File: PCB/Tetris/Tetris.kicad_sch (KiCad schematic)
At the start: 49 parts, among them J1 Power, J2 PWM, J3 Analog, J4 PWM, J5 Analog, J6 Communication, J7 Digital, M1 RGBMatrix, M2 RGBMatrix, SW1 SW_Push, SW2 SW_Push, SW3 SW_Push, SW4 SW_Push, SW5 SW_Push, SW6 SW_Push, SW7 SW_Push, U1 74HC595, U2 74HC595

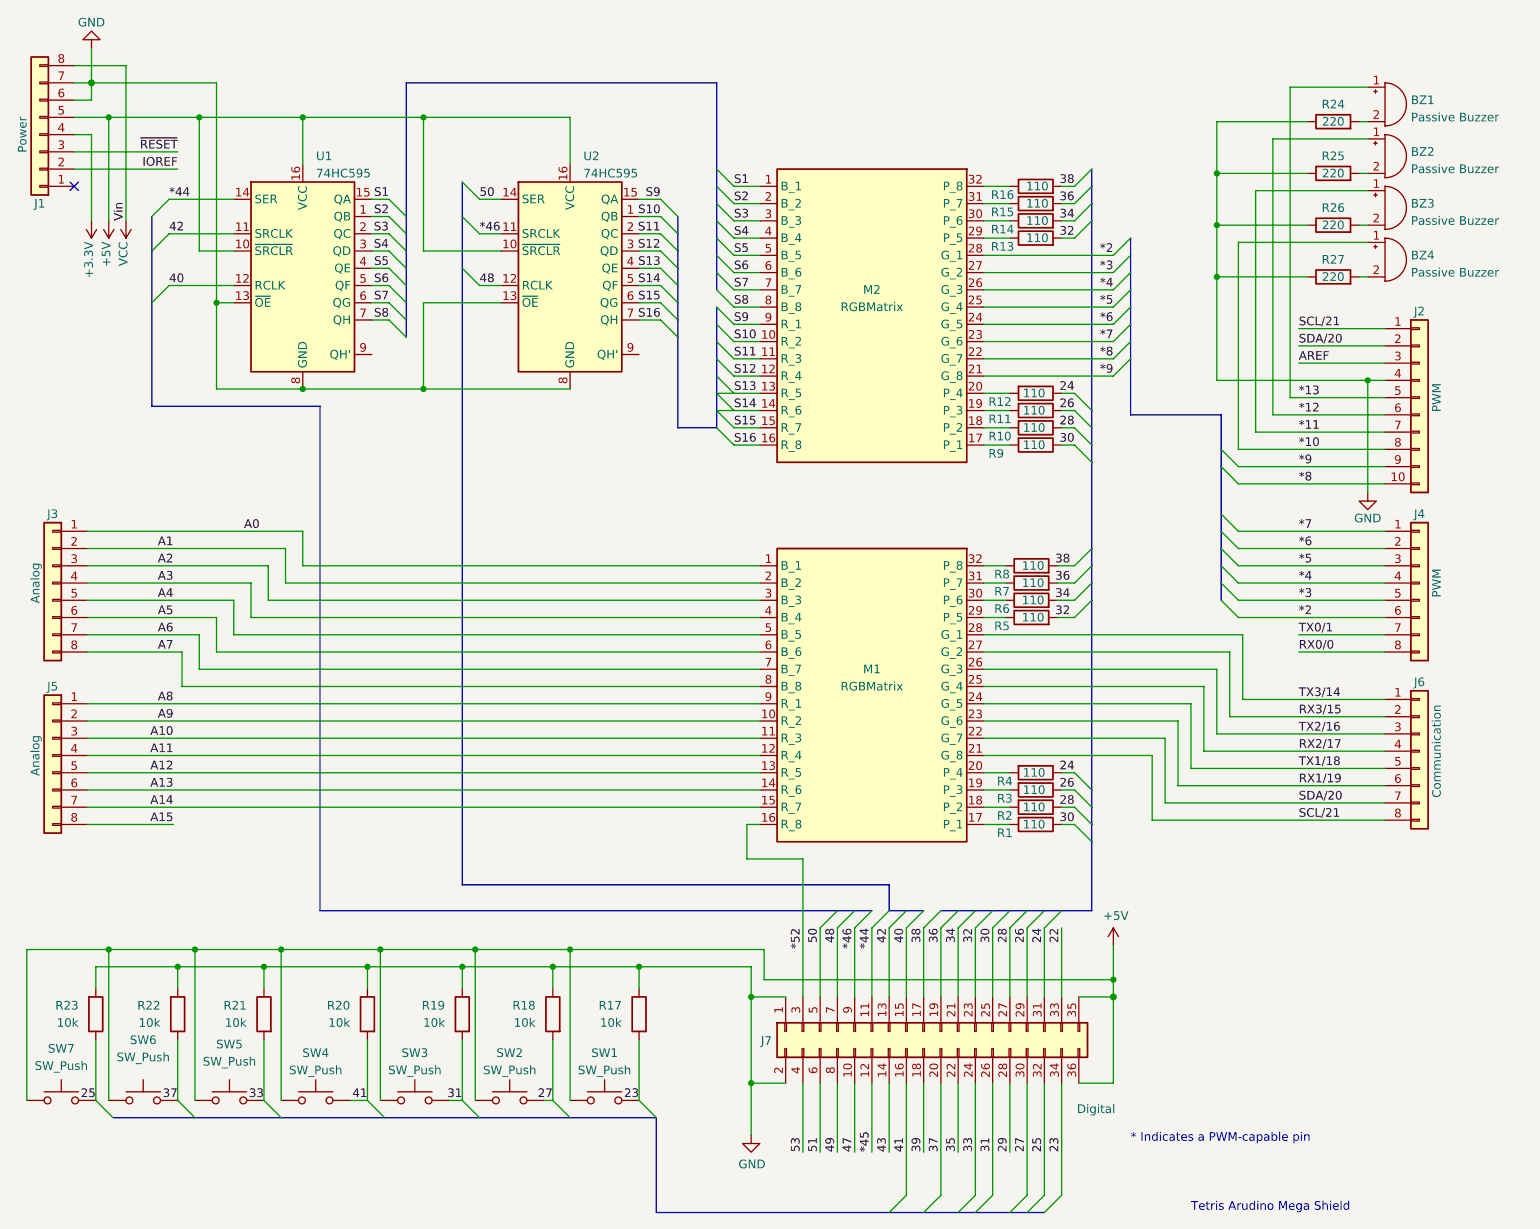
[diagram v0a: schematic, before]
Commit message: sync hcnages
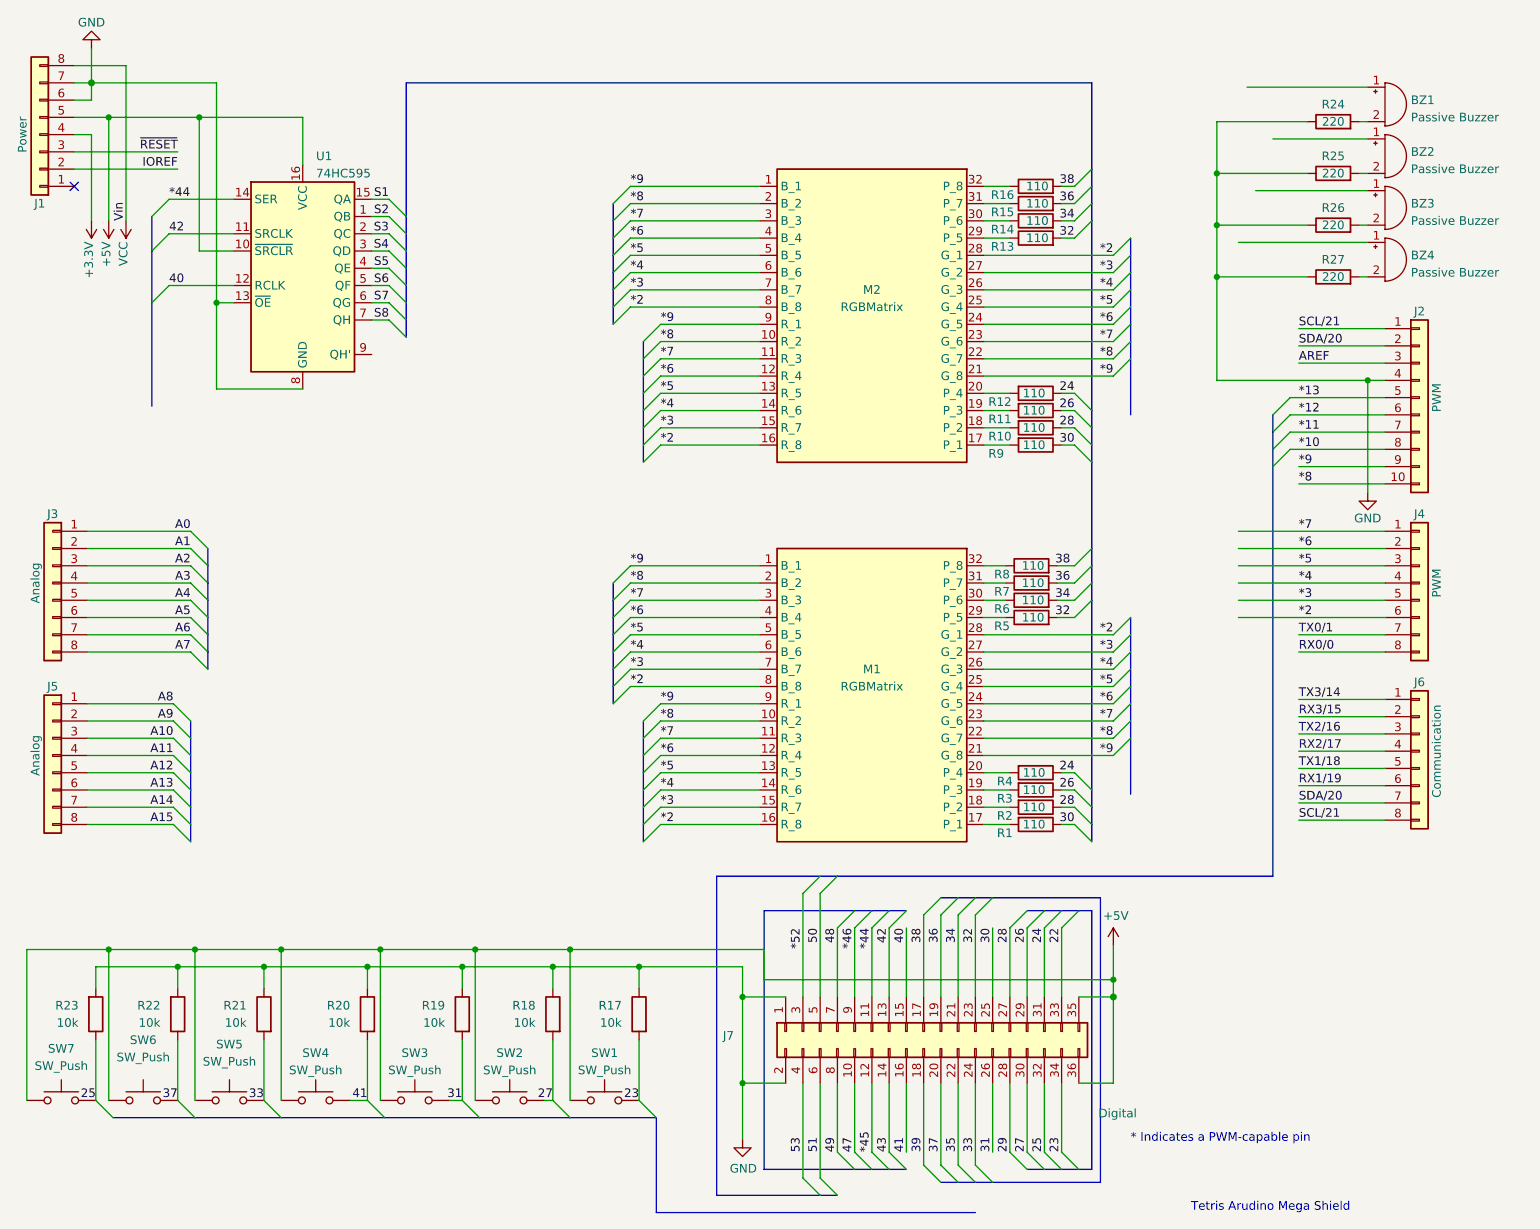
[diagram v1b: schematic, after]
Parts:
- removed U2: 74HC595, Package_DIP:DIP-16_W7.62mm_Socket_LongPads, symbol 74xx:74HC595
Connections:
- net S10 is gone; now on net *8: M2.10 (R_2)
- net S11 is gone; now on net *7: M2.11 (R_3)
- net S12 is gone; now on net *6: M2.12 (R_4)
- net S13 is gone; now on net *5: M2.13 (R_5)
- net S14 is gone; now on net *4: M2.14 (R_6)
- net S15 is gone; now on net *3: M2.15 (R_7)
- net S16 is gone; now on net *2: M2.16 (R_8)
- net S9 is gone; now on net *9: M2.9 (R_1)
- net *10: no longer BZ4.1 (-)
- net *11: no longer BZ3.1 (-)
- net *12: no longer BZ2.1 (-)
- net *13: no longer BZ1.1 (-)
- net *2: now also M1.16 (R_8), M1.28 (G_1), M1.8 (B_8), M2.8 (B_8)
- net *3: now also M1.15 (R_7), M1.27 (G_2), M1.7 (B_7), M2.7 (B_7)
- net *4: now also M1.14 (R_6), M1.26 (G_3), M1.6 (B_6), M2.6 (B_6)
- net *5: now also M1.13 (R_5), M1.25 (G_4), M1.5 (B_5), M2.5 (B_5)
- net *52: no longer M1.16 (R_8)
- net *6: now also M1.12 (R_4), M1.24 (G_5), M1.4 (B_4), M2.4 (B_4)
- net *7: now also M1.11 (R_3), M1.23 (G_6), M1.3 (B_3), M2.3 (B_3)
- net *8: now also M1.10 (R_2), M1.2 (B_2), M1.22 (G_7), M2.2 (B_2)
- net *9: now also M1.1 (B_1), M1.21 (G_8), M1.9 (R_1), M2.1 (B_1)
- net A0: no longer M1.1 (B_1)
- net A1: no longer M1.2 (B_2)
- net A10: no longer M1.11 (R_3)
- net A11: no longer M1.12 (R_4)
- net A12: no longer M1.13 (R_5)
- net A13: no longer M1.14 (R_6)
- net A14: no longer M1.15 (R_7)
- net A2: no longer M1.3 (B_3)
- net A3: no longer M1.4 (B_4)
- net A4: no longer M1.5 (B_5)
- net A5: no longer M1.6 (B_6)
- net A6: no longer M1.7 (B_7)
- net A7: no longer M1.8 (B_8)
- net A8: no longer M1.9 (R_1)
- net A9: no longer M1.10 (R_2)
- net RX1/19: no longer M1.23 (G_6)
- net RX2/17: no longer M1.25 (G_4)
- net RX3/15: no longer M1.27 (G_2)
- net S1: no longer M2.1 (B_1)
- net S2: no longer M2.2 (B_2)
- net S3: no longer M2.3 (B_3)
- net S4: no longer M2.4 (B_4)
- net S5: no longer M2.5 (B_5)
- net S6: no longer M2.6 (B_6)
- net S7: no longer M2.7 (B_7)
- net S8: no longer M2.8 (B_8)
- net SCL/21: no longer M1.21 (G_8)
- net SDA/20: no longer M1.22 (G_7)
- net TX1/18: no longer M1.24 (G_5)
- net TX2/16: no longer M1.26 (G_3)
- net TX3/14: no longer M1.28 (G_1)

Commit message: MASSIVE PROGRESS
Redesign PCB to use ports
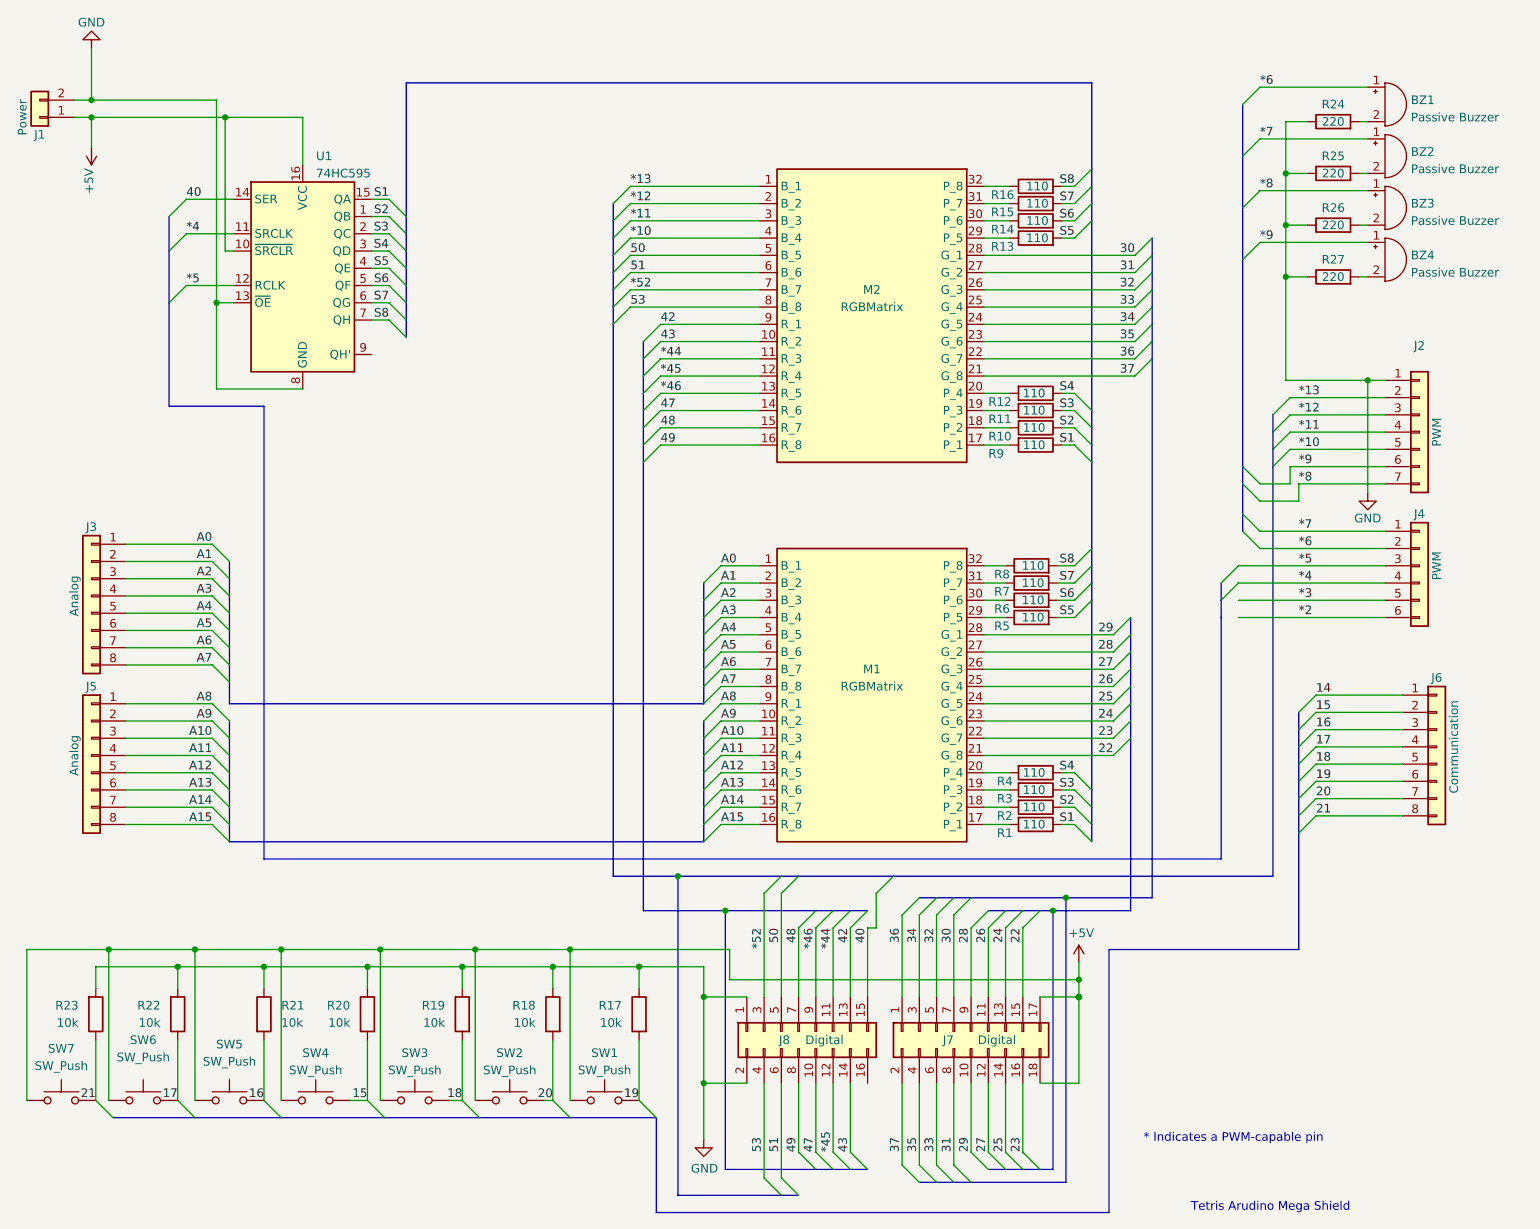
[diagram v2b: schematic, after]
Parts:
- added J8: Digital, Connector_PinHeader_2.54mm:PinHeader_2x08_P2.54mm_Vertical, symbol Connector_Generic:Conn_02x08_Odd_Even
- J1: footprint Connector_PinHeader_2.54mm:PinHeader_1x08_P2.54mm_Vertical -> Connector_PinHeader_2.54mm:PinHeader_1x02_P2.54mm_Vertical; symbol Connector_Generic:Conn_01x08 -> Connector_Generic:Conn_01x02
- J2: footprint Connector_PinHeader_2.54mm:PinHeader_1x10_P2.54mm_Vertical -> Connector_PinHeader_2.54mm:PinHeader_1x07_P2.54mm_Vertical; symbol Connector_Generic:Conn_01x10 -> Connector_Generic:Conn_01x07
- J4: footprint Connector_PinHeader_2.54mm:PinHeader_1x08_P2.54mm_Vertical -> Connector_PinHeader_2.54mm:PinHeader_1x06_P2.54mm_Vertical; symbol Connector_Generic:Conn_01x08 -> Connector_Generic:Conn_01x06
- J7: footprint Connector_PinHeader_2.54mm:PinHeader_2x18_P2.54mm_Vertical -> Connector_PinHeader_2.54mm:PinHeader_2x09_P2.54mm_Vertical; symbol Connector_Generic:Conn_02x18_Odd_Even -> Connector_Generic:Conn_02x09_Odd_Even
- R1, R10, R11, R12, R2, R24, R25, R26, R27, R3, R4, R5, R6, R7, R8, R9: footprint Resistor_THT:R_Axial_DIN0207_L6.3mm_D2.5mm_P10.16mm_Horizontal -> RGBMatrix:R_Axial_DIN0207_L6.3mm_D2.5mm_P12.40mm_Horizontal
- R17, R18: footprint Resistor_THT:R_Axial_DIN0207_L6.3mm_D2.5mm_P10.16mm_Horizontal -> Resistor_THT:R_Axial_DIN0207_L6.3mm_D2.5mm_P7.62mm_Horizontal
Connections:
- net 39 is gone; now on net +5V: J7.18 (Pin_18)
- net AREF is gone; now on net *12: J2.3 (Pin_3)
- net IOREF is gone; now on net GND: J1.2 (Pin_2)
- net RX3/15 is gone; now on net 15: J6.2 (Pin_2)
- net *10: now also J2.5 (Pin_5), M2.4 (B_4); no longer J2.8 (Pin_8)
- net *11: now also J2.4 (Pin_4), M2.3 (B_3); no longer J2.7 (Pin_7)
- net *12: now also M2.2 (B_2); no longer J2.6 (Pin_6)
- net *13: now also J2.2 (Pin_2), M2.1 (B_1); no longer J2.5 (Pin_5)
- net *2: no longer M1.16 (R_8), M1.28 (G_1), M1.8 (B_8), M2.16 (R_8), M2.28 (G_1), M2.8 (B_8)
- net *3: no longer M1.15 (R_7), M1.27 (G_2), M1.7 (B_7), M2.15 (R_7), M2.27 (G_2), M2.7 (B_7)
- net *4: now also U1.11 (SRCLK); no longer M1.14 (R_6), M1.26 (G_3), M1.6 (B_6), M2.14 (R_6), M2.26 (G_3), M2.6 (B_6)
- net *44: now also M2.11 (R_3), J8.11 (Pin_11); no longer J7.11 (Pin_11), U1.14 (SER)
- net *45: now also M2.12 (R_4), J8.12 (Pin_12); no longer J7.12 (Pin_12)
- net *46: now also M2.13 (R_5), J8.9 (Pin_9); no longer J7.9 (Pin_9)
- net *5: now also U1.12 (RCLK); no longer M1.13 (R_5), M1.25 (G_4), M1.5 (B_5), M2.13 (R_5), M2.25 (G_4), M2.5 (B_5)
- net *52: now also M2.7 (B_7), J8.3 (Pin_3); no longer J7.3 (Pin_3)
- net *6: now also BZ1.1 (-); no longer M1.12 (R_4), M1.24 (G_5), M1.4 (B_4), M2.12 (R_4), M2.24 (G_5), M2.4 (B_4)
- net *7: now also BZ2.1 (-); no longer M1.11 (R_3), M1.23 (G_6), M1.3 (B_3), M2.11 (R_3), M2.23 (G_6), M2.3 (B_3)
- net *8: now also BZ3.1 (-), J2.7 (Pin_7); no longer J2.10 (Pin_10), M1.10 (R_2), M1.2 (B_2), M1.22 (G_7), M2.10 (R_2), M2.2 (B_2), M2.22 (G_7)
- net *9: now also BZ4.1 (-), J2.6 (Pin_6); no longer J2.9 (Pin_9), M1.1 (B_1), M1.21 (G_8), M1.9 (R_1), M2.1 (B_1), M2.21 (G_8), M2.9 (R_1)
- net +5V: now also J1.1 (Pin_1), J7.17 (Pin_17); no longer J1.5 (Pin_5), J7.35 (Pin_35), J7.36 (Pin_36)
- net 22: now also J7.15 (Pin_15), M1.21 (G_8); no longer J7.33 (Pin_33)
- net 23: now also J7.16 (Pin_16), M1.22 (G_7); no longer J7.34 (Pin_34), R17.2, SW1.1
- net 24: now also J7.13 (Pin_13), M1.23 (G_6); no longer J7.31 (Pin_31), R12.1, R4.1
- net 25: now also J7.14 (Pin_14), M1.24 (G_5); no longer J7.32 (Pin_32), R23.1, SW7.1
- net 26: now also J7.11 (Pin_11), M1.25 (G_4); no longer J7.29 (Pin_29), R11.1, R3.1
- net 27: now also J7.12 (Pin_12), M1.26 (G_3); no longer J7.30 (Pin_30), R18.2, SW2.1
- net 28: now also J7.9 (Pin_9), M1.27 (G_2); no longer J7.27 (Pin_27), R10.1, R2.1
- net 29: now also J7.10 (Pin_10), M1.28 (G_1); no longer J7.28 (Pin_28)
- net 30: now also J7.7 (Pin_7), M2.28 (G_1); no longer J7.25 (Pin_25), R1.1, R9.1
- net 31: now also J7.8 (Pin_8), M2.27 (G_2); no longer J7.26 (Pin_26), R19.2, SW3.1
- net 32: now also J7.5 (Pin_5), M2.26 (G_3); no longer J7.23 (Pin_23), R13.2, R5.2
- net 33: now also J7.6 (Pin_6), M2.25 (G_4); no longer J7.24 (Pin_24), R21.2, SW5.1
- net 34: now also J7.3 (Pin_3), M2.24 (G_5); no longer J7.21 (Pin_21), R14.2, R6.2
- net 35: now also J7.4 (Pin_4), M2.23 (G_6); no longer J7.22 (Pin_22)
- net 36: now also J7.1 (Pin_1), M2.22 (G_7); no longer J7.19 (Pin_19), R15.2, R7.2
- net 37: now also J7.2 (Pin_2), M2.21 (G_8); no longer J7.20 (Pin_20), R22.1, SW6.1
- net 40: now also U1.14 (SER), J8.15 (Pin_15); no longer J7.15 (Pin_15), U1.12 (RCLK)
- net 42: now also M2.9 (R_1), J8.13 (Pin_13); no longer J7.13 (Pin_13), U1.11 (SRCLK)
- net 43: now also M2.10 (R_2), J8.14 (Pin_14); no longer J7.14 (Pin_14)
- net 47: now also M2.14 (R_6), J8.10 (Pin_10); no longer J7.10 (Pin_10)
- net 48: now also M2.15 (R_7), J8.7 (Pin_7); no longer J7.7 (Pin_7)
- net 49: now also M2.16 (R_8), J8.8 (Pin_8); no longer J7.8 (Pin_8)
- net 50: now also M2.5 (B_5), J8.5 (Pin_5); no longer J7.5 (Pin_5)
- net 51: now also M2.6 (B_6), J8.6 (Pin_6); no longer J7.6 (Pin_6)
- net 53: now also M2.8 (B_8), J8.4 (Pin_4); no longer J7.4 (Pin_4)
- net A0: now also M1.1 (B_1)
- net A1: now also M1.2 (B_2)
- net A10: now also M1.11 (R_3)
- net A11: now also M1.12 (R_4)
- net A12: now also M1.13 (R_5)
- net A13: now also M1.14 (R_6)
- net A14: now also M1.15 (R_7)
- net A15: now also M1.16 (R_8)
- net A2: now also M1.3 (B_3)
- net A3: now also M1.4 (B_4)
- net A4: now also M1.5 (B_5)
- net A5: now also M1.6 (B_6)
- net A6: now also M1.7 (B_7)
- net A7: now also M1.8 (B_8)
- net A8: now also M1.9 (R_1)
- net A9: now also M1.10 (R_2)
- net GND: now also J2.1 (Pin_1), J8.1 (Pin_1), J8.2 (Pin_2); no longer J1.6 (Pin_6), J1.7 (Pin_7), J2.4 (Pin_4), J7.1 (Pin_1), J7.2 (Pin_2)
- net S1: now also R1.1, R9.1
- net S2: now also R10.1, R2.1
- net S3: now also R11.1, R3.1
- net S4: now also R12.1, R4.1
- net S5: now also R13.2, R5.2
- net S6: now also R14.2, R6.2
- net S7: now also R15.2, R7.2
- net S8: now also R16.2, R8.2
- removed net +3V3: J1.4 (Pin_4)
- removed net 38: J7.17 (Pin_17), R16.2, R8.2
- net 41 renamed 15
- net 15: no longer J7.16 (Pin_16)
- removed net RX0/0: J4.8 (Pin_8)
- net RX1/19 renamed 19
- net 19: now also R17.2, SW1.1
- net RX2/17 renamed 17
- net 17: now also R22.1, SW6.1
- net SCL/21 renamed 21
- net 21: now also R23.1, SW7.1; no longer J2.1 (Pin_1)
- net SDA/20 renamed 20
- net 20: now also R18.2, SW2.1; no longer J2.2 (Pin_2)
- removed net TX0/1: J4.7 (Pin_7)
- net TX1/18 renamed 18
- net 18: now also R19.2, SW3.1
- net TX2/16 renamed 16
- net 16: now also R21.2, SW5.1
- net TX3/14 renamed 14
- removed net VCC: J1.8 (Pin_8)
- removed net ~{RESET}: J1.3 (Pin_3)
- no-connect marks 1 -> 0
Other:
- moved on the sheet: J3, J5, J6
